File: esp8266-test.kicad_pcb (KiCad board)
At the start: 2 copper layers, 58.3 x 48.8 mm, 37 parts, among them J1 TEENSY-LC, J28 HEADER-MALE-1POS-TH-1x01, J29 HEADER-MALE-1POS-TH-1x01, J30 HEADER-MALE-1POS-TH-1x01, J31 HEADER-MALE-1POS-TH-1x01

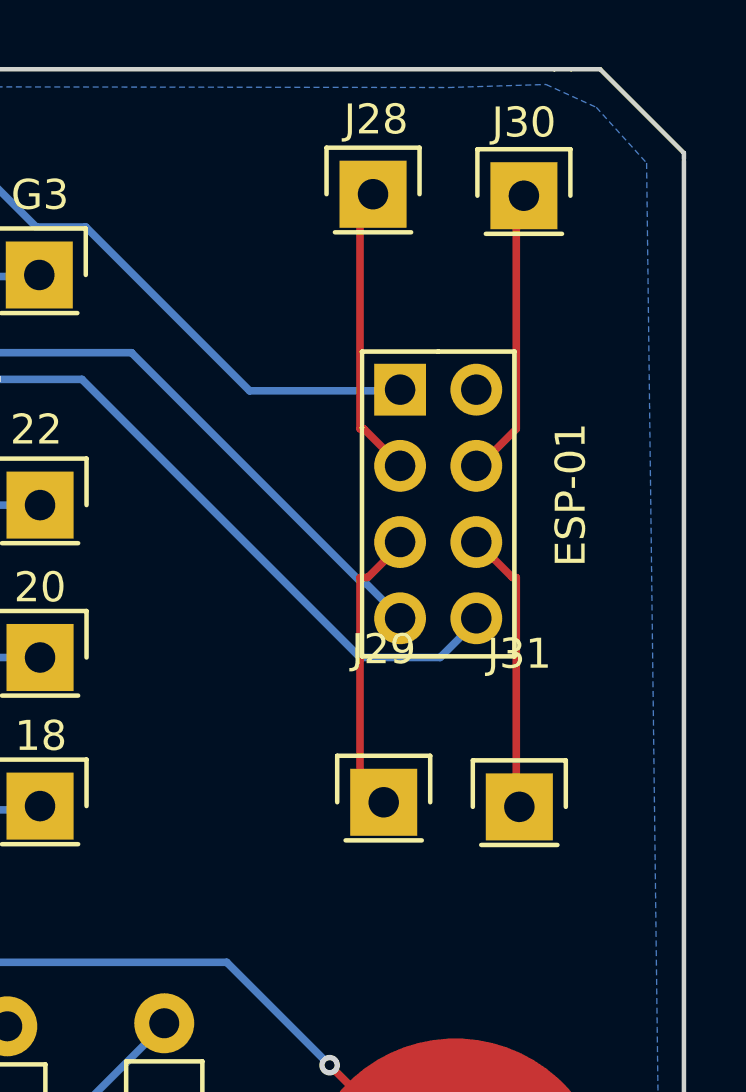
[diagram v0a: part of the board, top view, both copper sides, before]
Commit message: update layout
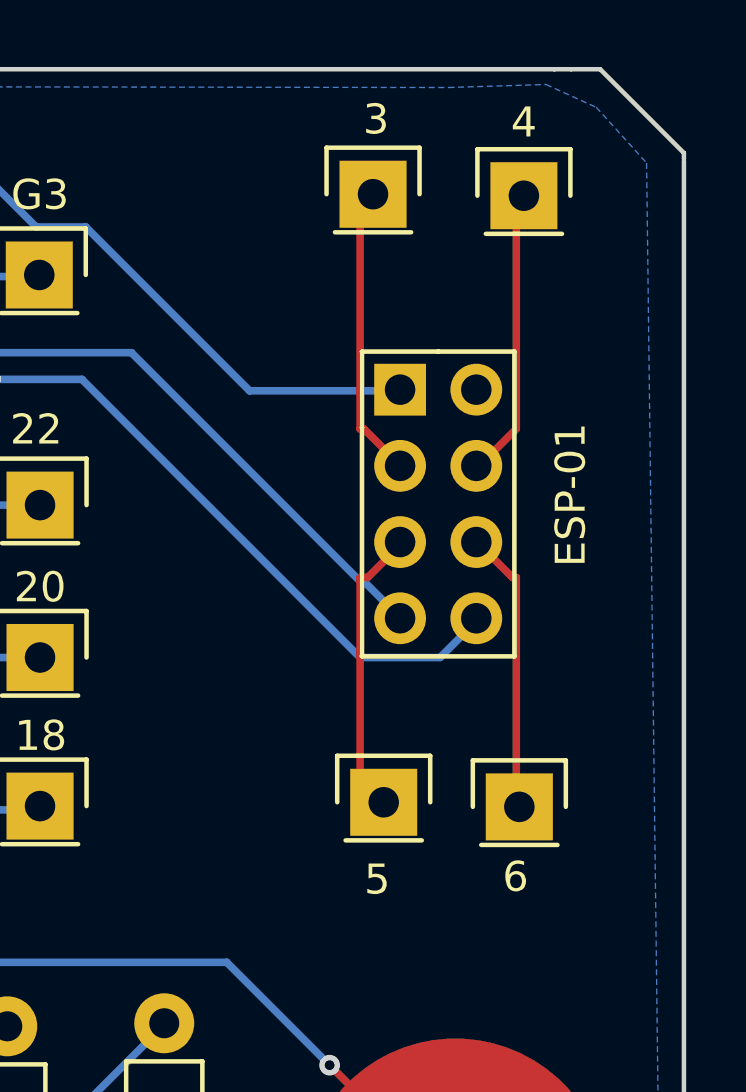
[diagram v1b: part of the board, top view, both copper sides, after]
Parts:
- renumbered J28 to 3, J30 to 4, J29 to 5, J31 to 6
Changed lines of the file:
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@@
     (links 41)
     (no_connects 0)
-    (area 83.693 55.626 178.435 123.19)
+    (area 83.778238 55.5738 178.510001 123.265001)
     (thickness 1.6)
     (drawings 36)
@@
     (descr "Through hole pin header")
     (tags "pin header")
-    (fp_text reference J28 (at 0.1016 -2.4892) (layer F.SilkS)
+    (fp_text reference 3 (at 0.1016 -2.4892) (layer F.SilkS)
       (effects (font (size 1 1) (thickness 0.15)))
     )
@@
     (descr "Through hole pin header")
     (tags "pin header")
-    (fp_text reference J29 (at 0 -5.1) (layer F.SilkS)
+    (fp_text reference 5 (at -0.2159 2.5781) (layer F.SilkS)
       (effects (font (size 1 1) (thickness 0.15)))
     )
@@
     (descr "Through hole pin header")
     (tags "pin header")
-    (fp_text reference J30 (at 0 -2.4384) (layer F.SilkS)
+    (fp_text reference 4 (at 0 -2.4384) (layer F.SilkS)
       (effects (font (size 1 1) (thickness 0.15)))
     )
@@
     (descr "Through hole pin header")
     (tags "pin header")
-    (fp_text reference J31 (at 0 -5.1) (layer F.SilkS)
-      (effects (font (size 1 1) (thickness 0.15)))
-    )
+    (fp_text reference 6 (at -0.127 2.3368) (layer F.SilkS)
+      (effects (font (size 1 1) (thickness 0.15)))
+    )
